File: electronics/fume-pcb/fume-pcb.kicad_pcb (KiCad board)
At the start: 2 copper layers, 120 x 90 mm, 40 parts, among them J1 PWR Conn, J2 2_Wire_conn, J3 4_Wire_conn, J4 3_Wire_conn, J5 Ref_conn, Q1 STP12PF06, Q2 2N3904, Q3 2N3906, Q4 2N3904, Q5 IRFZ44N, SW1 SW_SEL

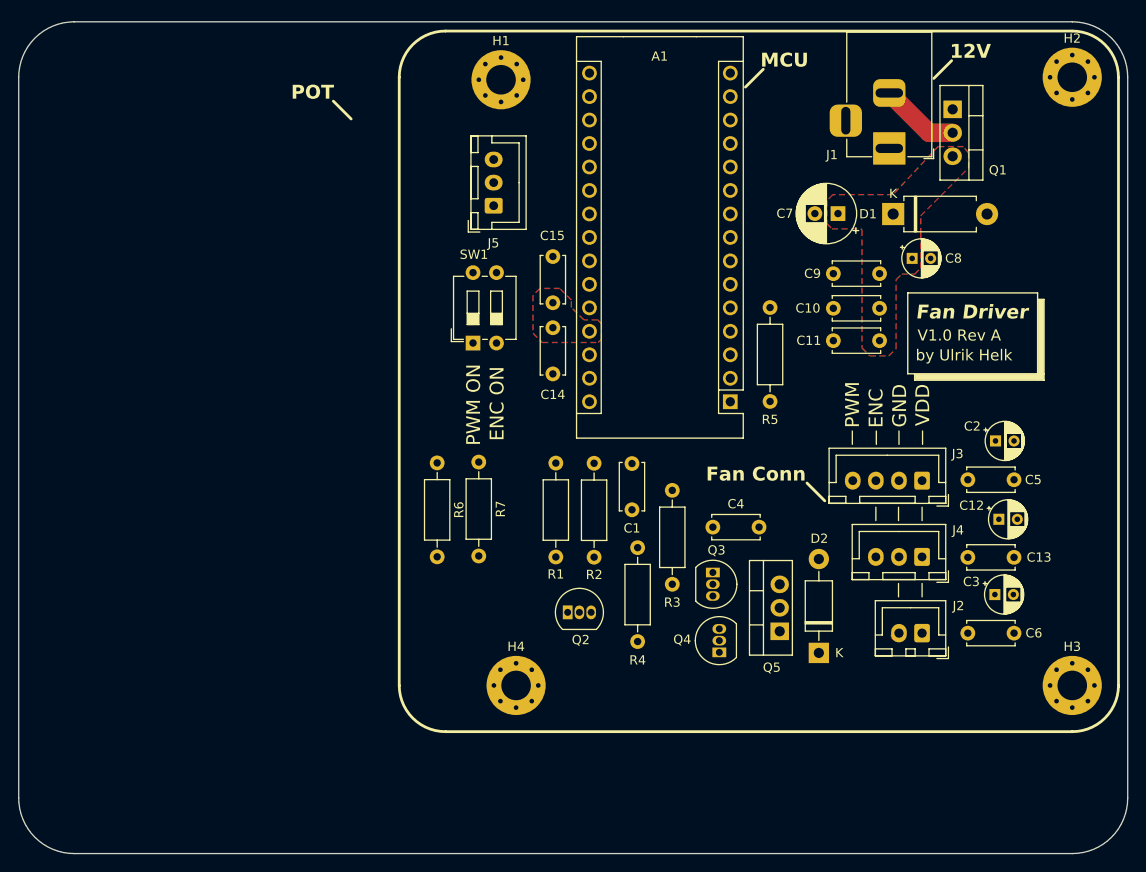
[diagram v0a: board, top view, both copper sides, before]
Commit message: Update
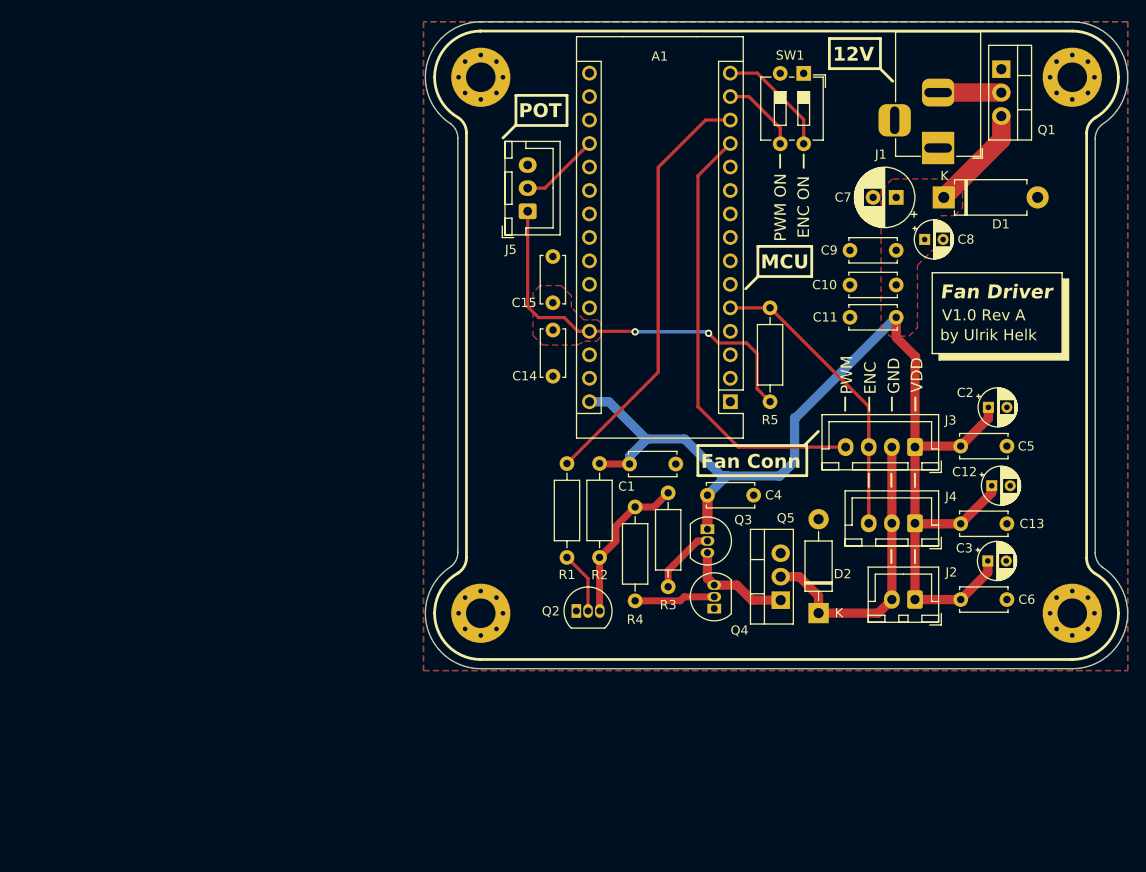
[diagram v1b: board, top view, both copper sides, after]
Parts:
- removed R6, R7: 10k, Resistor_THT:R_Axial_DIN0207_L6.3mm_D2.5mm_P10.16mm_Horizontal
- added REF**: WEEE-Logo_5.6x8mm_SilkScreen, Symbol:WEEE-Logo_5.6x8mm_SilkScreen, B.Cu at (189.3, 113.3)
- moved SW1 46.2 mm to (169.9, 55.6), turned to -90 degrees
- moved H4 8.69 mm to (135.0, 114.0)
- moved H3 7.81 mm to (199.0, 114.0)
- moved Q1 6.83 mm to (191.3, 55.1)
- moved C7 6.54 mm to (179.9, 69.0)
- moved D1 5.76 mm to (185.1, 69.0)
- moved J1 5.29 mm to (184.5, 63.7)
- moved Q4 4.77 mm to (160.3, 113.5)
- moved Q3 4.72 mm to (159.5, 104.9)
- moved R4 4.41 mm to (151.7, 102.5)
- moved D2 4.31 mm to (171.6, 114.0)
- moved J5 3.73 mm to (140.1, 70.5)
- moved C12 3.72 mm to (190.3, 100.2)
- moved J2 3.72 mm to (182.0, 112.5)
- moved J3 3.72 mm to (182.0, 96.0)
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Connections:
- A1 pad 14: unconnected-(A1-D11-Pad14) -> /ON_PWM
- A1 pad 15: unconnected-(A1-D12-Pad15) -> /ON_ENC
- SW1 pad 1: +5V -> GND
- SW1 pad 2: +5V -> GND
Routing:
- net +12V: track 0.08 -> 133.8 mm
- net /PWM_FAN: track 0.00 -> 47.7 mm
- net /PWM_MOS: track 0.00 -> 46.1 mm
- net +5V: track 0.00 -> 43.1 mm, vias 0 -> 2
- net /ENC_FAN: track 0.00 -> 32.0 mm
- net /GND_FAN: track 0.39 -> 31.8 mm
- net Net-(Q2-C): track 0.00 -> 17.1 mm
- net /ON_ENC: track 0.00 -> 12.6 mm
- net Net-(Q3-C): track 0.00 -> 11.7 mm
- net Net-(Q4-B): track 0.00 -> 8.74 mm
- net /REF_FAN: track 0.00 -> 8.69 mm
- net /ON_PWM: track 0.00 -> 8.52 mm
- net Net-(Q3-B): track 0.00 -> 7.33 mm
- net Net-(Q2-B): track 0.00 -> 6.73 mm
- net /VIN: track 8.64 -> 6.84 mm
- added copper zone on B.Cu, net GND
- added copper zone on F.Cu, net GND
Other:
- board size 120 x 90 mm -> 76 x 70 mm

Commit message: Almost done with PCB
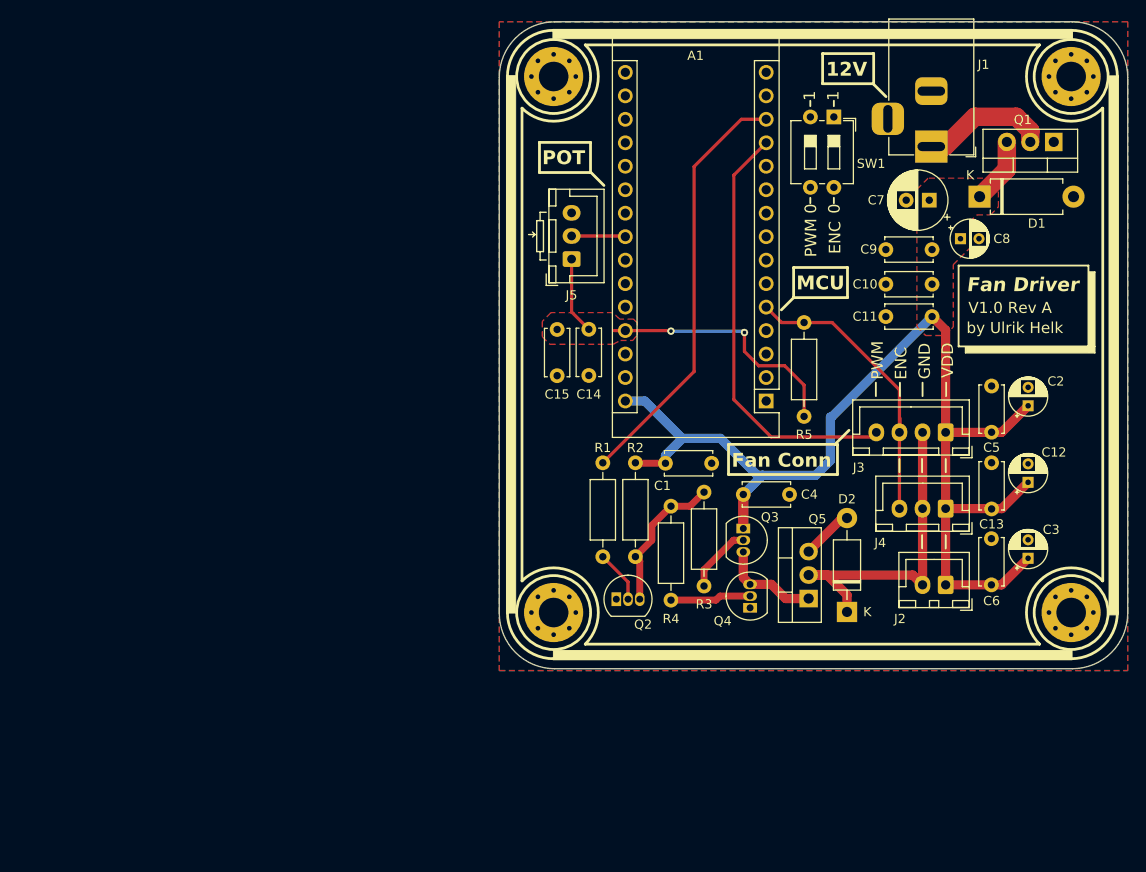
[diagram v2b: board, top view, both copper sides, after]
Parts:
- moved Q1 9.71 mm to (197.0, 63.0), turned to 180 degrees
- moved H1 7.88 mm to (142.9, 55.9)
- moved H4 7.88 mm to (142.9, 113.9)
- moved J5 7.02 mm to (144.8, 75.7)
- moved SW1 5.74 mm to (173.2, 60.3)
- moved Q2 4.51 mm to (149.7, 112.5)
- moved C3 4.37 mm to (194.2, 108.1), turned to 90 degrees
- moved C2 4.30 mm to (194.2, 91.6), turned to 90 degrees
- moved R5 4.01 mm to (170.0, 92.7)
- moved C12 3.95 mm to (194.2, 99.8), turned to 90 degrees
- moved C10 3.88 mm to (183.8, 78.4)
- moved C11 3.88 mm to (183.8, 81.9)
- moved C9 3.88 mm to (183.8, 74.6)
- moved R1 3.88 mm to (148.2, 97.7)
- moved R4 3.88 mm to (155.6, 102.4)
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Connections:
- A1 pad 19: /REF_FAN -> unconnected-(A1-A0-Pad19)
- A1 pad 23: unconnected-(A1-A4-Pad23) -> /REF_FAN
- J1 pad 1: GND -> /VIN
- J1 pad 2: /VIN -> GND
- J1 pad 3: (no net) -> GND
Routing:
- net /ON_ENC: track 12.6 -> 0.00 mm
- net /ON_PWM: track 8.52 -> 0.24 mm
- net +5V: track 43.1 -> 36.0 mm
- net /VIN: track 6.84 -> 13.9 mm
- net +12V: track 133.8 -> 127.1 mm
- net GND: track 0.00 -> 5.65 mm
- net /GND_FAN: track 31.8 -> 36.1 mm
- net /REF_FAN: track 8.69 -> 5.85 mm
- net /PWM_FAN: track 47.7 -> 46.5 mm
- net Net-(Q2-C): track 17.1 -> 16.1 mm
- net Net-(Q2-B): track 6.73 -> 5.72 mm
- net Net-(Q3-C): track 11.7 -> 10.8 mm
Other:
- board size 76 x 70 mm -> 68 x 70 mm
- board text added: "0"
- board text added: "1"
- board text removed: "ENC ON"
- board text removed: "PWM ON"

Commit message: PCB ORDERED
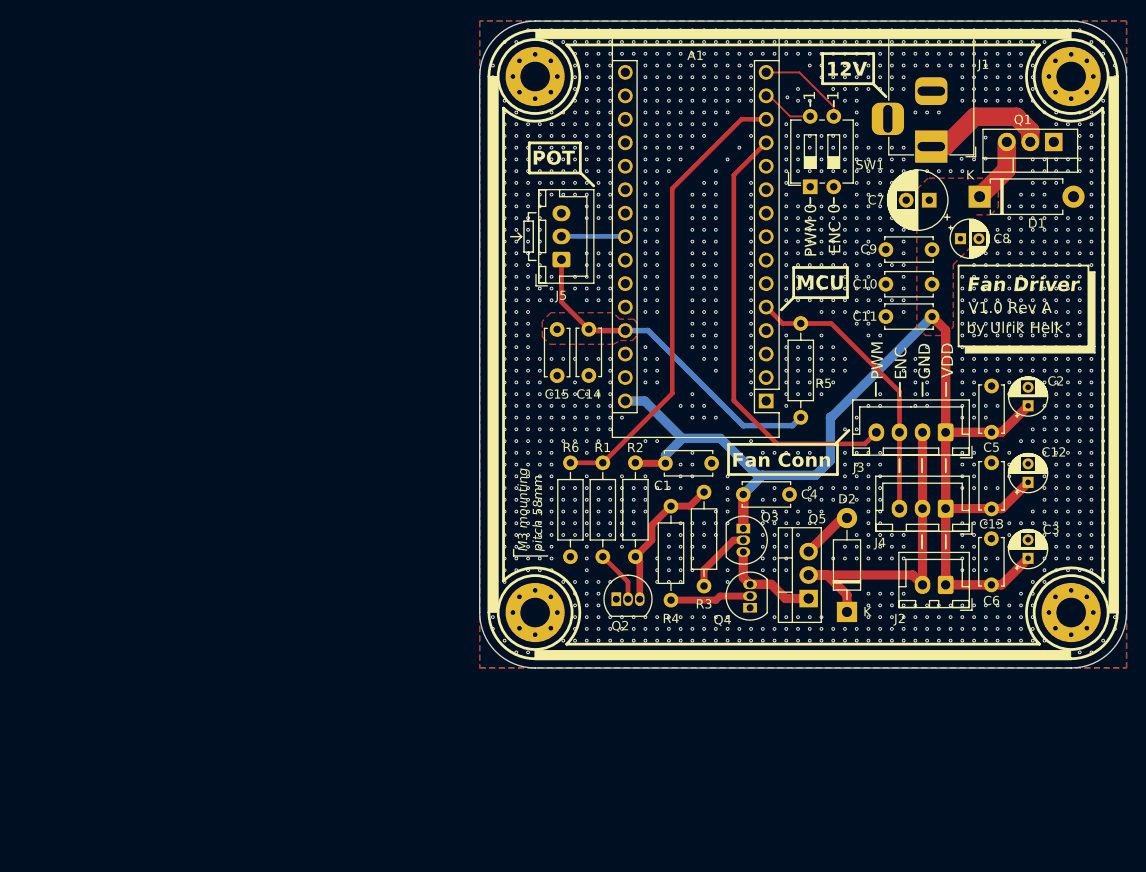
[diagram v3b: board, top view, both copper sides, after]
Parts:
- removed REF**: WEEE-Logo_5.6x8mm_SilkScreen, Symbol:WEEE-Logo_5.6x8mm_SilkScreen
- added G***: LOGO, 0_logo:fan_80x80mm, B.Cu at (170.0, 85.0)
- added R6: 10k, Resistor_THT:R_Axial_DIN0207_L6.3mm_D2.5mm_P10.16mm_Horizontal, F.Cu at (144.7, 107.9)
- moved SW1 7.98 mm to (170.7, 67.8), turned to 90 degrees
- moved H1 2.00 mm to (140.9, 55.9)
- moved H4 2.00 mm to (140.9, 113.9)
- moved J5 1.10 mm to (143.7, 75.7)
- moved R5 0.37 mm to (169.6, 92.8)
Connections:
- A1 pad 14: /ON_PWM -> /ON_ENC
- A1 pad 15: /ON_ENC -> /ON_PWM
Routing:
- net /ON_PWM: track 0.24 -> 9.89 mm
- net /ON_ENC: track 0.00 -> 5.94 mm
- net /PWM_MOS: track 46.1 -> 49.6 mm
- net /ENC_FAN: track 32.5 -> 30.9 mm
- net /REF_FAN: track 5.85 -> 7.17 mm
- net /PWM_FAN: track 46.5 -> 47.2 mm
- net +5V: track 36.0 -> 36.4 mm, vias 2 -> 0
- net GND: vias 0 -> 1727
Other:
- board size 68 x 70 mm -> 70 x 70 mm
- board text added: "M3 mounting pitch 58mm"
- board text added: "he1k 03/25"
